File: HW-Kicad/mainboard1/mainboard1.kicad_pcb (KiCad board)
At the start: 2 copper layers, 101 x 101 mm, 15 parts, among them J1 Conn_01x04_Male, J2 Conn_01x02_Male, J3 Conn_01x07_Male, J4 Conn_01x04_Male, J5 Conn_01x04_Male, J8 Conn_02x10_Odd_Even, U1 MCP1700-2802E_TO92, U2 ESP32-WROOM-E, U3 Mini360, U4 YAAJ_DCDC_StepDown_LM2596

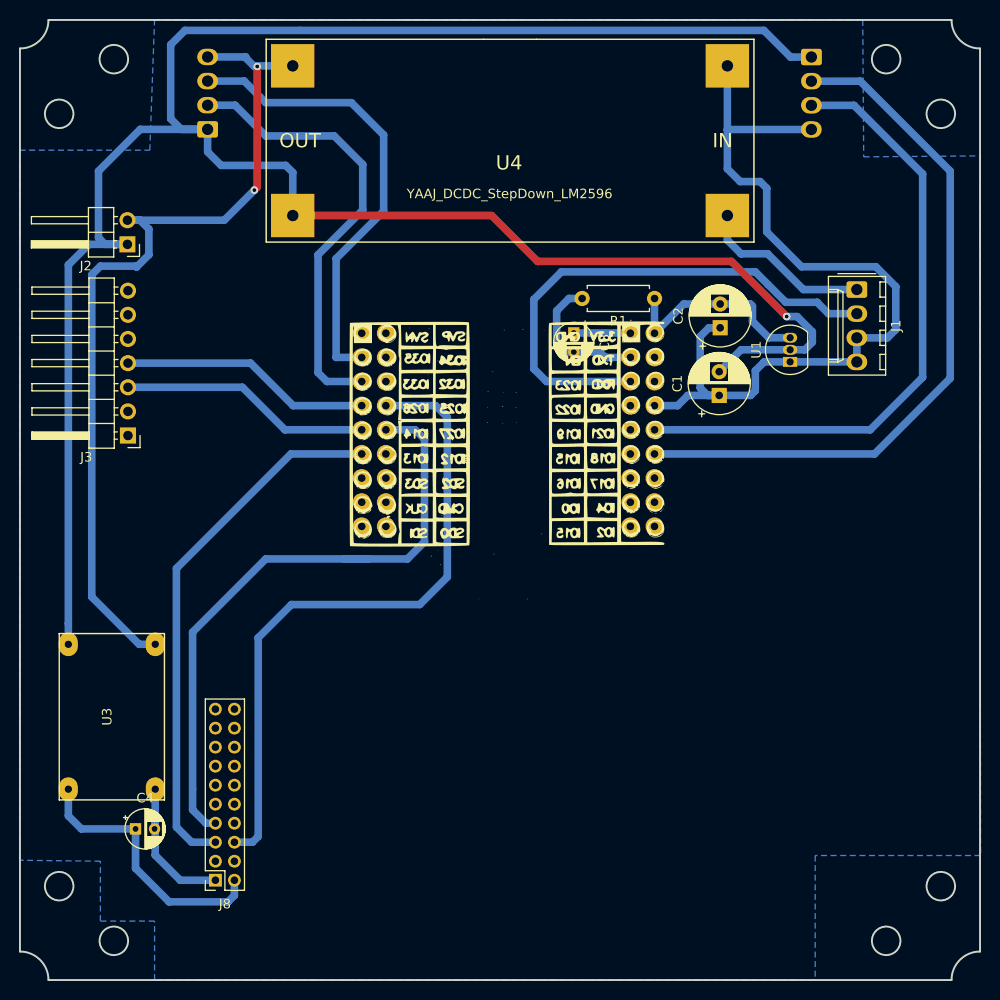
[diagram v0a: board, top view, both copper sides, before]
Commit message: importe nueva version de leo
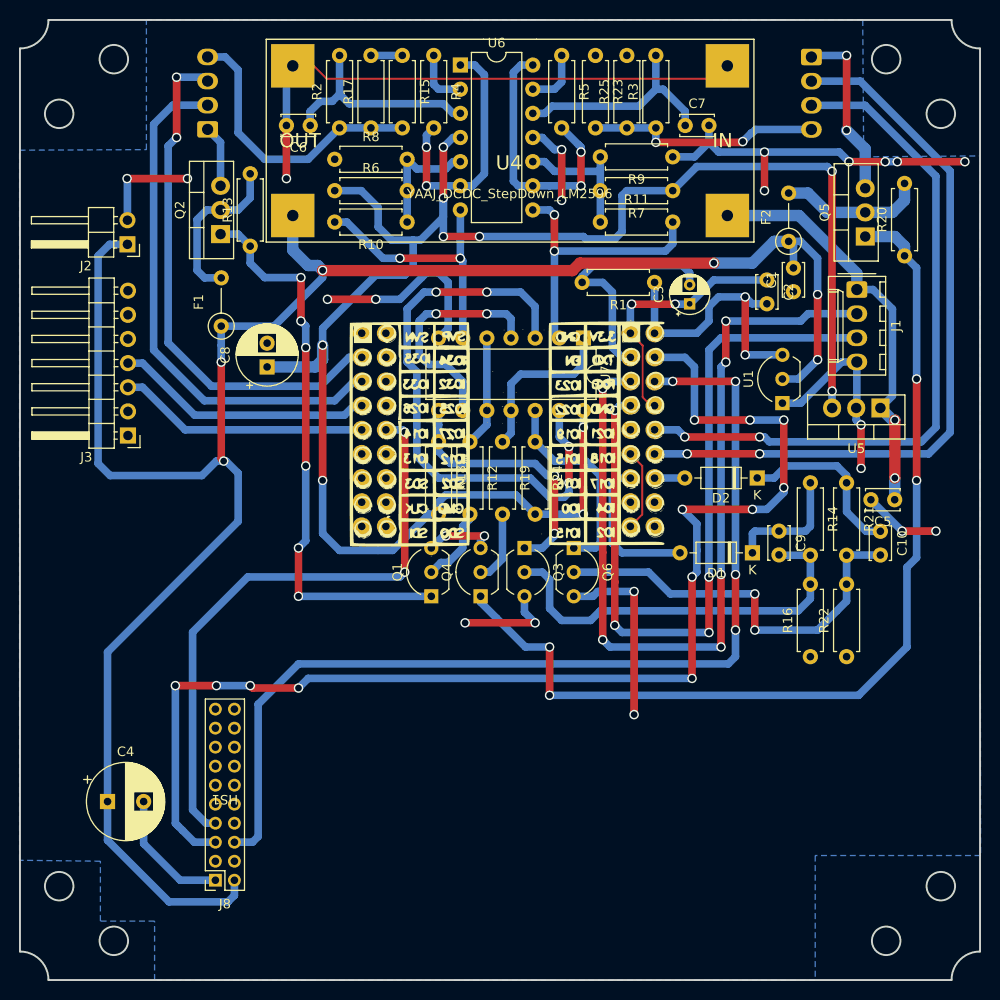
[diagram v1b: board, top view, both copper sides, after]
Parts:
- removed U3: Mini360, mini360:Mini360_step-down
- added C10: 100n, Capacitor_THT:C_Disc_D3.4mm_W2.1mm_P2.50mm, F.Cu at (206.8, 93.5)
- added C5: 100n, Capacitor_THT:C_Disc_D3.4mm_W2.1mm_P2.50mm, F.Cu at (208.3, 90.2)
- added C6: 100n, Capacitor_THT:C_Disc_D3.4mm_W2.1mm_P2.50mm, F.Cu at (146.8, 50.8)
- added C7: 100n, Capacitor_THT:C_Disc_D3.4mm_W2.1mm_P2.50mm, F.Cu at (186.2, 50.8)
- added C8: 100u, Capacitor_THT:CP_Radial_D6.3mm_P2.50mm, F.Cu at (142.2, 76.2)
- added C9: 100n, Capacitor_THT:C_Disc_D3.4mm_W2.1mm_P2.50mm, F.Cu at (196.1, 93.5)
- added D1: 1N4148, Diode_THT:D_DO-35_SOD27_P7.62mm_Horizontal, F.Cu at (193.3, 95.8)
- added D2: 1N4148, Diode_THT:D_DO-35_SOD27_P7.62mm_Horizontal, F.Cu at (193.8, 87.9)
- added F1: Polyfuse, Resistor_THT:R_Axial_DIN0207_L6.3mm_D2.5mm_P5.08mm_Vertical, F.Cu at (137.4, 71.9)
- added F2: Polyfuse, Resistor_THT:R_Axial_DIN0207_L6.3mm_D2.5mm_P5.08mm_Vertical, F.Cu at (197.1, 63.0)
- added HS1: Heatsink, Library:9xtend, F.Cu at (137.8, 121.2)
- added Q1: BC337, Package_TO_SOT_THT:TO-92_Inline_Wide, F.Cu at (159.5, 100.3)
- added Q2: IRF9540N, Package_TO_SOT_THT:TO-220-3_Vertical, F.Cu at (137.3, 62.2)
- added Q3: BC337, Package_TO_SOT_THT:TO-92_Inline_Wide, F.Cu at (169.3, 95.2)
- added Q4: BC337, Package_TO_SOT_THT:TO-92_Inline_Wide, F.Cu at (164.7, 100.3)
- added Q5: IRF9540N, Package_TO_SOT_THT:TO-220-3_Vertical, F.Cu at (205.2, 62.5)
- added Q6: BC337, Package_TO_SOT_THT:TO-92_Inline_Wide, F.Cu at (174.5, 95.2)
- added R10: 4.7k, Resistor_THT:R_Axial_DIN0207_L6.3mm_D2.5mm_P7.62mm_Horizontal, F.Cu at (157.0, 61.0)
- added R11: 4.7k, Resistor_THT:R_Axial_DIN0207_L6.3mm_D2.5mm_P7.62mm_Horizontal, F.Cu at (177.3, 61.0)
- added R12: 10k, Resistor_THT:R_Axial_DIN0207_L6.3mm_D2.5mm_P7.62mm_Horizontal, F.Cu at (163.6, 84.1)
- added R13: 10k, Resistor_THT:R_Axial_DIN0207_L6.3mm_D2.5mm_P7.62mm_Horizontal, F.Cu at (140.5, 63.5)
- added R14: 100k, Resistor_THT:R_Axial_DIN0207_L6.3mm_D2.5mm_P7.62mm_Horizontal, F.Cu at (199.4, 88.4)
- added R15: 1, Resistor_THT:R_Axial_DIN0207_L6.3mm_D2.5mm_P7.62mm_Horizontal, F.Cu at (156.5, 43.4)
- added R16: 10k, Resistor_THT:R_Axial_DIN0207_L6.3mm_D2.5mm_P7.62mm_Horizontal, F.Cu at (199.4, 106.7)
- added R17: 1, Resistor_THT:R_Axial_DIN0207_L6.3mm_D2.5mm_P7.62mm_Horizontal, F.Cu at (153.2, 51.1)
- added R18: 10k, Resistor_THT:R_Axial_DIN0207_L6.3mm_D2.5mm_P7.62mm_Horizontal, F.Cu at (160.3, 84.1)
- added R19: 10k, Resistor_THT:R_Axial_DIN0207_L6.3mm_D2.5mm_P7.62mm_Horizontal, F.Cu at (167.0, 84.1)
- added R2: 100k, Resistor_THT:R_Axial_DIN0207_L6.3mm_D2.5mm_P7.62mm_Horizontal, F.Cu at (149.9, 51.1)
- added R20: 10k, Resistor_THT:R_Axial_DIN0207_L6.3mm_D2.5mm_P7.62mm_Horizontal, F.Cu at (209.3, 64.5)
- added R21: 100k, Resistor_THT:R_Axial_DIN0207_L6.3mm_D2.5mm_P7.62mm_Horizontal, F.Cu at (203.2, 88.4)
- added R22: 10k, Resistor_THT:R_Axial_DIN0207_L6.3mm_D2.5mm_P7.62mm_Horizontal, F.Cu at (203.2, 106.7)
- added R23: 1, Resistor_THT:R_Axial_DIN0207_L6.3mm_D2.5mm_P7.62mm_Horizontal, F.Cu at (176.8, 43.4)
- added R24: 10k, Resistor_THT:R_Axial_DIN0207_L6.3mm_D2.5mm_P7.62mm_Horizontal, F.Cu at (170.4, 84.1)
- added R25: 1, Resistor_THT:R_Axial_DIN0207_L6.3mm_D2.5mm_P7.62mm_Horizontal, F.Cu at (180.1, 51.1)
- added R3: 100k, Resistor_THT:R_Axial_DIN0207_L6.3mm_D2.5mm_P7.62mm_Horizontal, F.Cu at (183.1, 51.1)
- added R4: 100k, Resistor_THT:R_Axial_DIN0207_L6.3mm_D2.5mm_P7.62mm_Horizontal, F.Cu at (159.8, 43.4)
- added R5: 100k, Resistor_THT:R_Axial_DIN0207_L6.3mm_D2.5mm_P7.62mm_Horizontal, F.Cu at (173.2, 43.4)
- added R6: 3.3k, Resistor_THT:R_Axial_DIN0207_L6.3mm_D2.5mm_P7.62mm_Horizontal, F.Cu at (149.4, 57.7)
- added R7: 3.3k, Resistor_THT:R_Axial_DIN0207_L6.3mm_D2.5mm_P7.62mm_Horizontal, F.Cu at (184.9, 57.7)
- added R8: 10k, Resistor_THT:R_Axial_DIN0207_L6.3mm_D2.5mm_P7.62mm_Horizontal, F.Cu at (149.4, 54.4)
- added R9: 10k, Resistor_THT:R_Axial_DIN0207_L6.3mm_D2.5mm_P7.62mm_Horizontal, F.Cu at (184.9, 54.1)
- added U5: LM7805_TO220, Package_TO_SOT_THT:TO-220-3_Vertical, F.Cu at (206.8, 80.5)
- added U6: LM324, Package_DIP:DIP-14_W7.62mm, F.Cu at (162.6, 44.4)
- added U7: HEF4093B, Package_DIP:DIP-14_W7.62mm, F.Cu at (175.5, 73.2)
- C1, C2: value 100u -> 100n; footprint Capacitor_THT:CP_Radial_D6.3mm_P2.50mm -> Capacitor_THT:C_Disc_D3.4mm_W2.1mm_P2.50mm
- C4: value 100uF -> 470uF; footprint Capacitor_THT:CP_Radial_D4.0mm_P2.00mm -> Capacitor_THT:CP_Radial_D8.0mm_P3.80mm
- U1: footprint Package_TO_SOT_THT:TO-92_Inline -> Package_TO_SOT_THT:TO-92_Inline_Wide
- moved C1 13.4 mm to (197.6, 68.3)
- moved C3 12.6 mm to (186.7, 69.6), turned to 90 degrees
- moved C2 7.03 mm to (194.8, 67.1), turned to -90 degrees
- moved U1 4.42 mm to (196.4, 80.0)
- moved C4 4.12 mm to (125.5, 121.9)
- moved R1 1.69 mm to (183.0, 67.3)
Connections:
- C4 pad 1: Net-(C4-Pad1) -> VBAT
- C4 pad 2: Net-(C4-Pad2) -> GND
- J4 pad 1: VBAT -> VCC_protect_1
- J4 pad 4: GND -> GND_protect_1
- J5 pad 1: VBAT -> VCC_protect_2
- J5 pad 4: GND -> GND_protect_2
- J8 pad 1: Net-(C4-Pad2) -> GND
- J8 pad 2: Net-(C4-Pad1) -> VBAT
- U2 pad 27: unconnected-(U2-Pad27) -> uC_activation_FF1
- U2 pad 28: unconnected-(U2-Pad28) -> uC_activation_FF2
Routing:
- net +5V: track 0.00 -> 188.3 mm, vias 0 -> 10
- net xtendRX: track 0.00 -> 131.6 mm, vias 0 -> 12
- net xtendTX: track 0.00 -> 106.4 mm, vias 0 -> 4
- net Net-(Q4-Pad1): track 0.00 -> 102.3 mm, vias 0 -> 4
- net paracaidas: track 0.00 -> 80.5 mm, vias 0 -> 4
- net unconnected-(U2-Pad10): track 70.0 -> 0.00 mm
- net Net-(U7-Pad13): track 0.00 -> 61.1 mm, vias 0 -> 4
- net GND: track 189.4 -> 248.8 mm, vias 2 -> 25
- net Net-(Q1-Pad1): track 0.00 -> 59.4 mm, vias 0 -> 6
- net unconnected-(U2-Pad16): track 56.4 -> 0.00 mm
- net Net-(C10-Pad2): track 0.00 -> 43.1 mm, vias 0 -> 2
- net Net-(C9-Pad2): track 0.00 -> 42.8 mm
- net abortSig: track 55.0 -> 91.0 mm, vias 0 -> 6
- net FF_R2: track 0.00 -> 30.7 mm, vias 0 -> 2
- net GND_protect_1: track 0.00 -> 30.2 mm
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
